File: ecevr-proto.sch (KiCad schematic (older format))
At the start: 30 parts, among them SW1 SW_Push

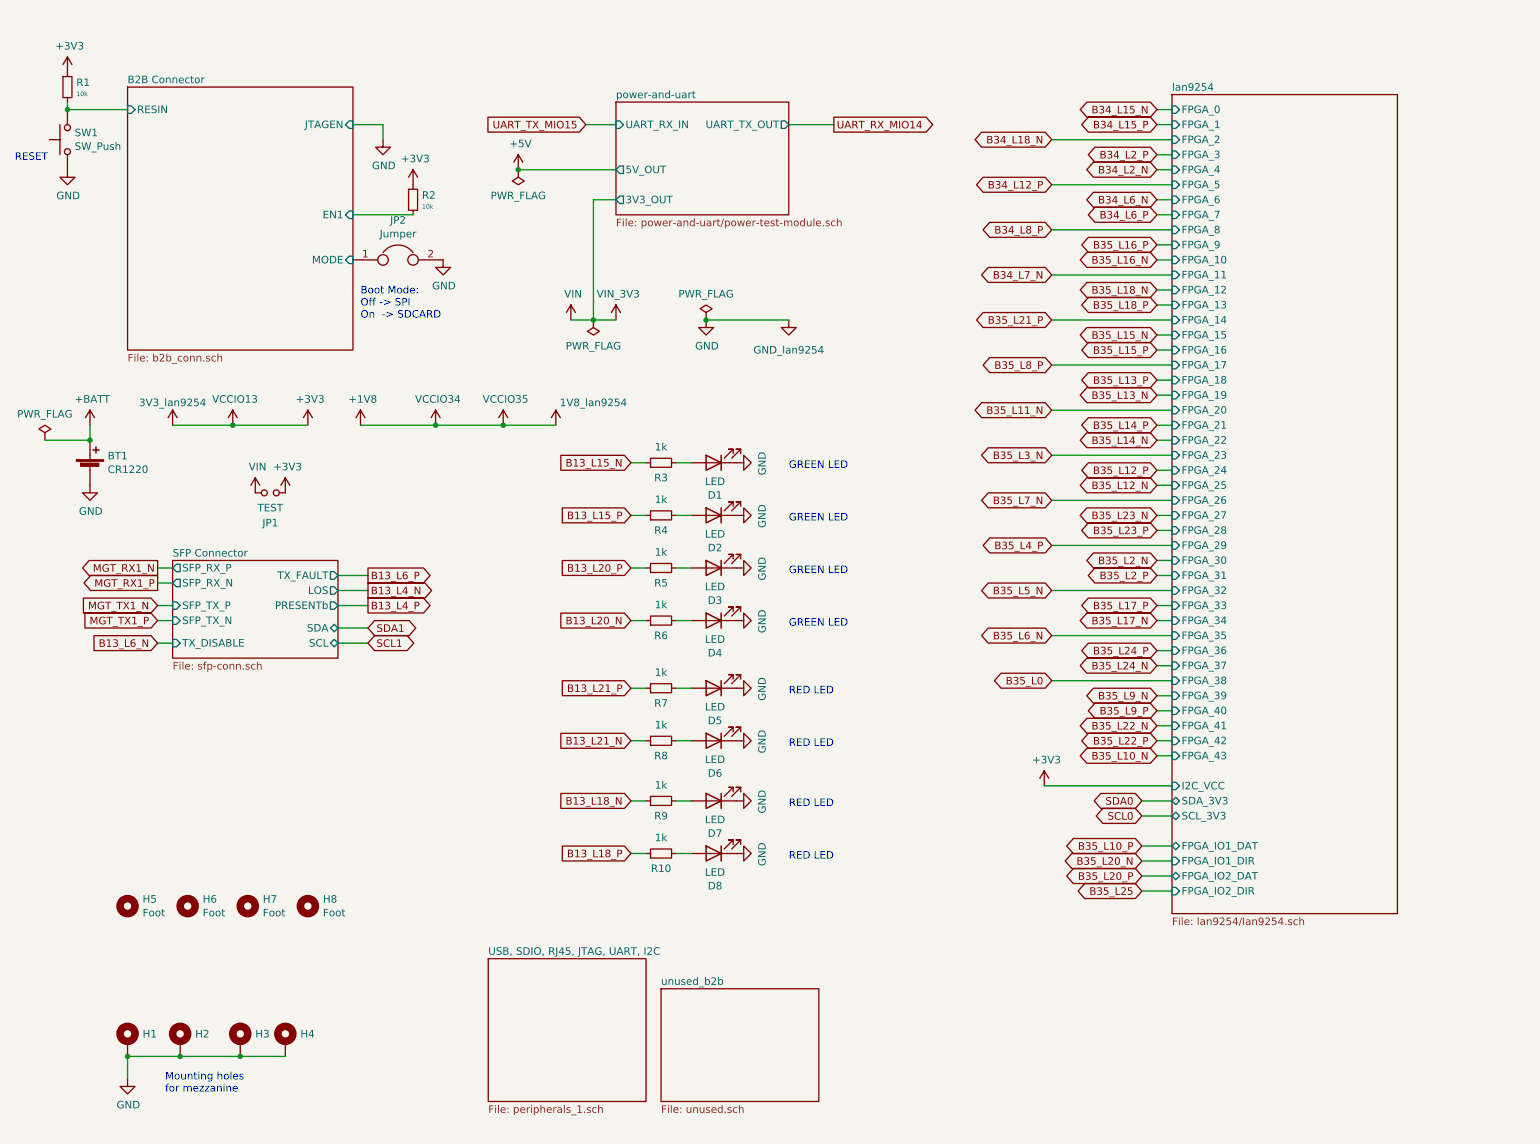
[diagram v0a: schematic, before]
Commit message: WIP: (save)
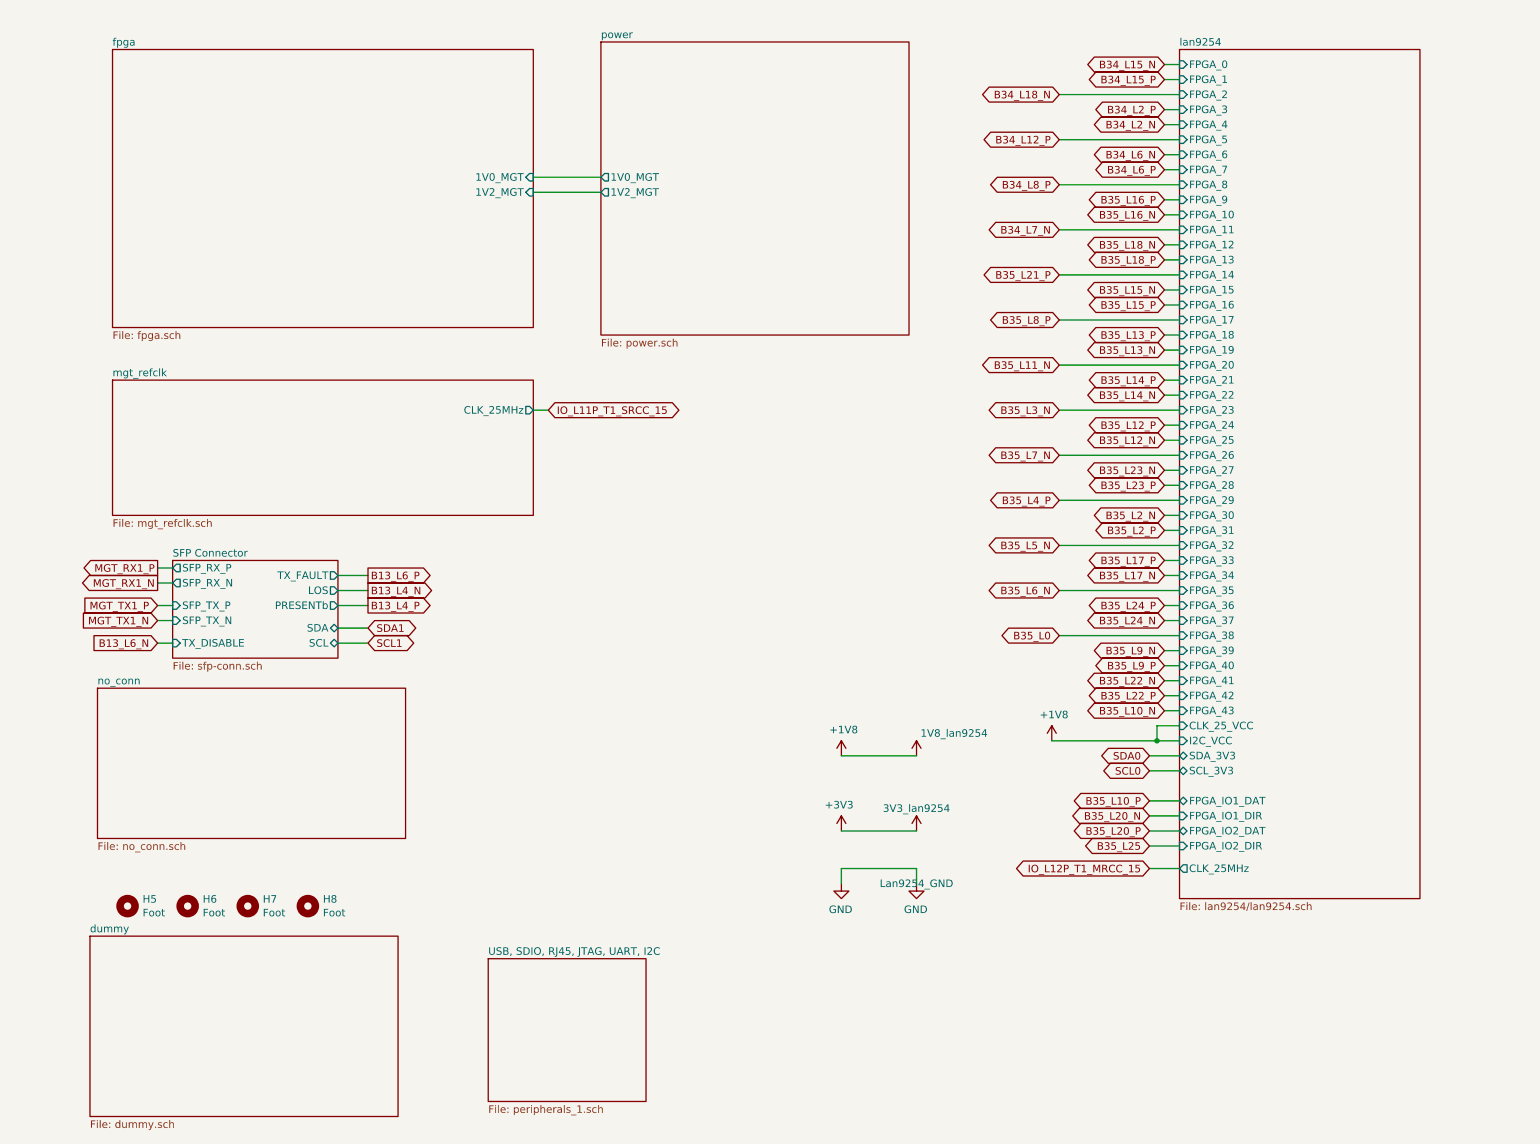
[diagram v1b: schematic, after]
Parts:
- removed BT1: CR1220, Battery:BatteryHolder_Keystone_500, symbol Device:Battery_Cell
- removed D1, D2, D3, D4, D5, D6, D7, D8: LED, LED_SMD:LED_0603_1608Metric, symbol Device:LED
- removed H1, H2, H3, H4: MountingHole_Pad, MountingHole:MountingHole_3.2mm_M3_ISO14580_Pad_TopBottom, symbol Mechanical:MountingHole_Pad
- removed JP1: TEST, Connector_PinHeader_2.54mm:PinHeader_1x02_P2.54mm_Vertical, symbol Device:Jumper_NO_Small
- removed JP2: Jumper, Connector_PinHeader_2.54mm:PinHeader_1x02_P2.54mm_Vertical, symbol Device:Jumper
- removed R1, R2: 10k, Resistor_SMD:R_0603_1608Metric, symbol trigbox:R10k
- removed R10, R3, R4, R5, R6, R7, R8, R9: 1k, Resistor_SMD:R_0603_1608Metric, symbol Device:R_Small
- removed SW1: SW_Push, Button_Switch_SMD:SW_SPST_PTS810, symbol Switch:SW_Push
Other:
- note removed: "Boot Mode:\nOff -> SPI\nOn -> SDCARD"
- note removed: "GREEN LED"
- note removed: "Mounting holes\nfor mezzanine"
- note removed: "RED LED"
- note removed: "RESET"

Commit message: WIP: point before we change to OSH/relaxed process
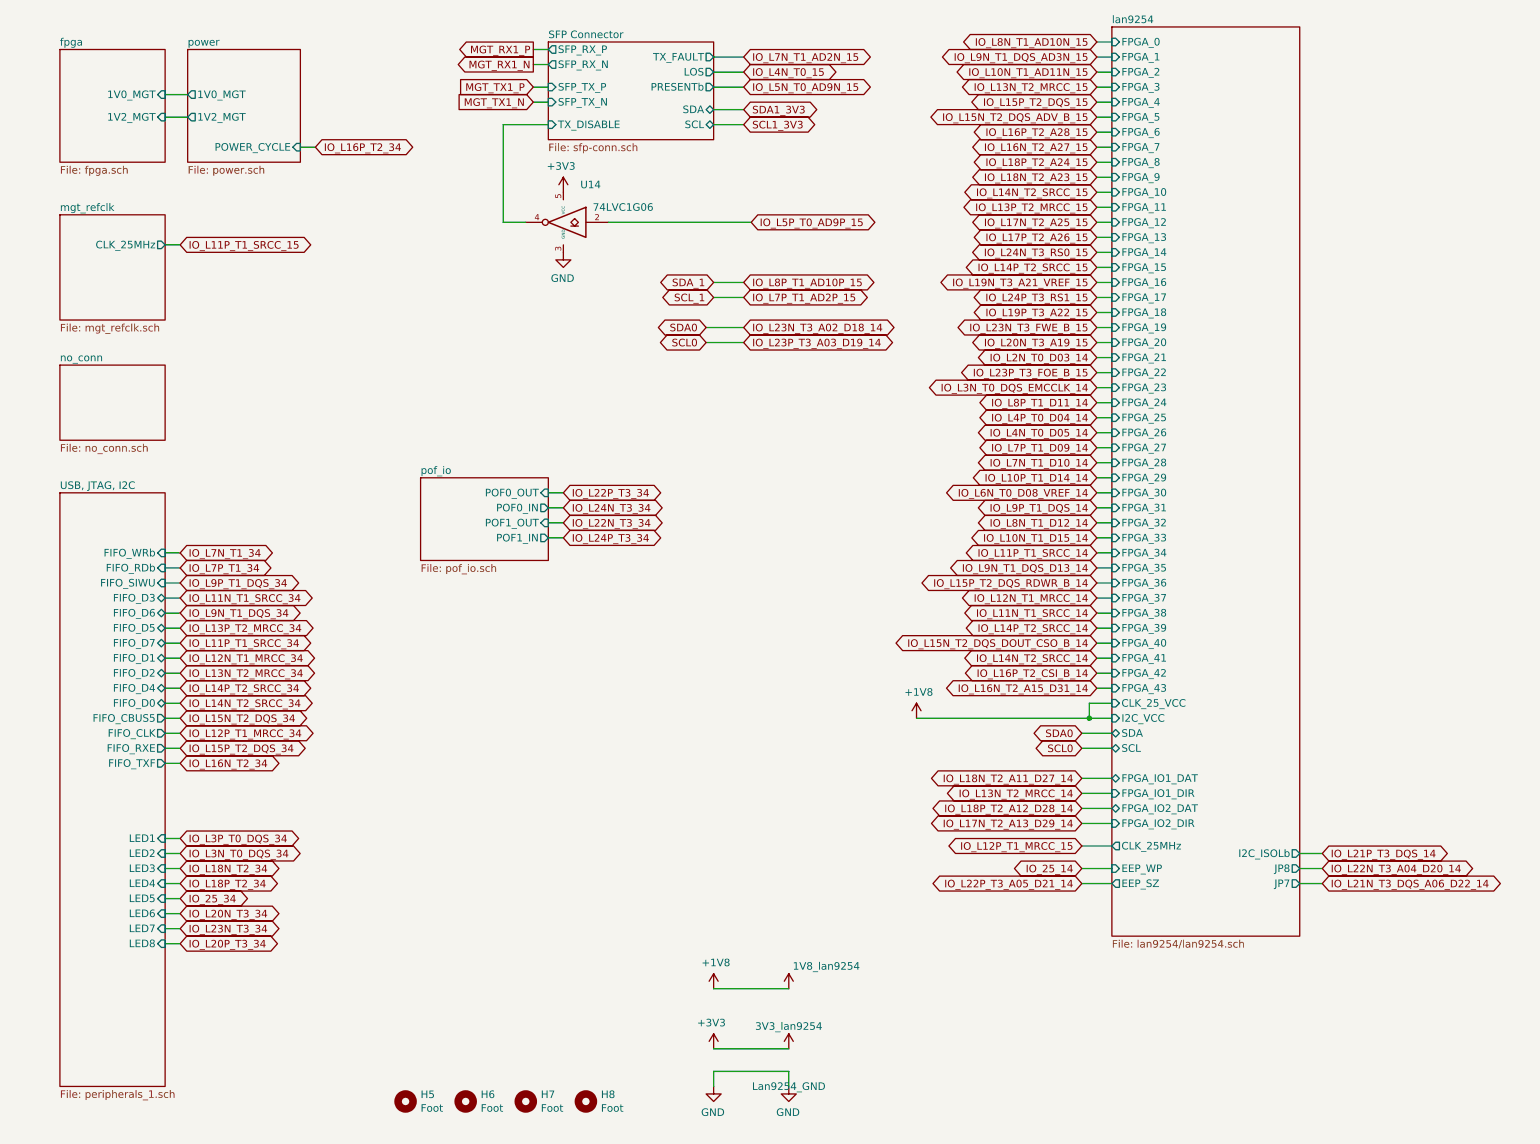
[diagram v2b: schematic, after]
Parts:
- added U14: 74LVC1G06, proj_footprints:SOT-5x3, symbol fmc:74LVC1G06
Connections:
- net +3V3: now also U14.5 (VCC)
- net GND: now also U14.3 (GND)
- new net IO_L5P_T0_AD9P_15: U14.2
- new net SFP Connector/TX_DISABLE: U14.4
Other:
- moved on the sheet: H5, H6, H7, H8
